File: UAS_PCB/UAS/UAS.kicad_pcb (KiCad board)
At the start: 2 copper layers, 50.8 x 47.6 mm, 17 parts, among them J1 SM02B-PASS-TBT, J2 SM02B-PASS-TBT, J3 SM02B-PASS-TBT, J4 SM02B-PASS-TBT, U1 JST-7-Pin, U10 UAS-rescue_7.5V-2.4A-Converte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, U11 JST-3-Pin, U12 Signal-Pad, U13 Signal-Pad, U2 5A-5V-Converter, U3 500mA-5V-Converter, U4 12V-StepUp-Converter, U5 TB6612FNG-Dual-Motor-Driver, U6 16_Pad_2x8_Set-UAS-cache, U7 UAS-rescue_JST-4-Pin-UAS-cache, U8 JST-7-Pin, U9 JST-3-Pin

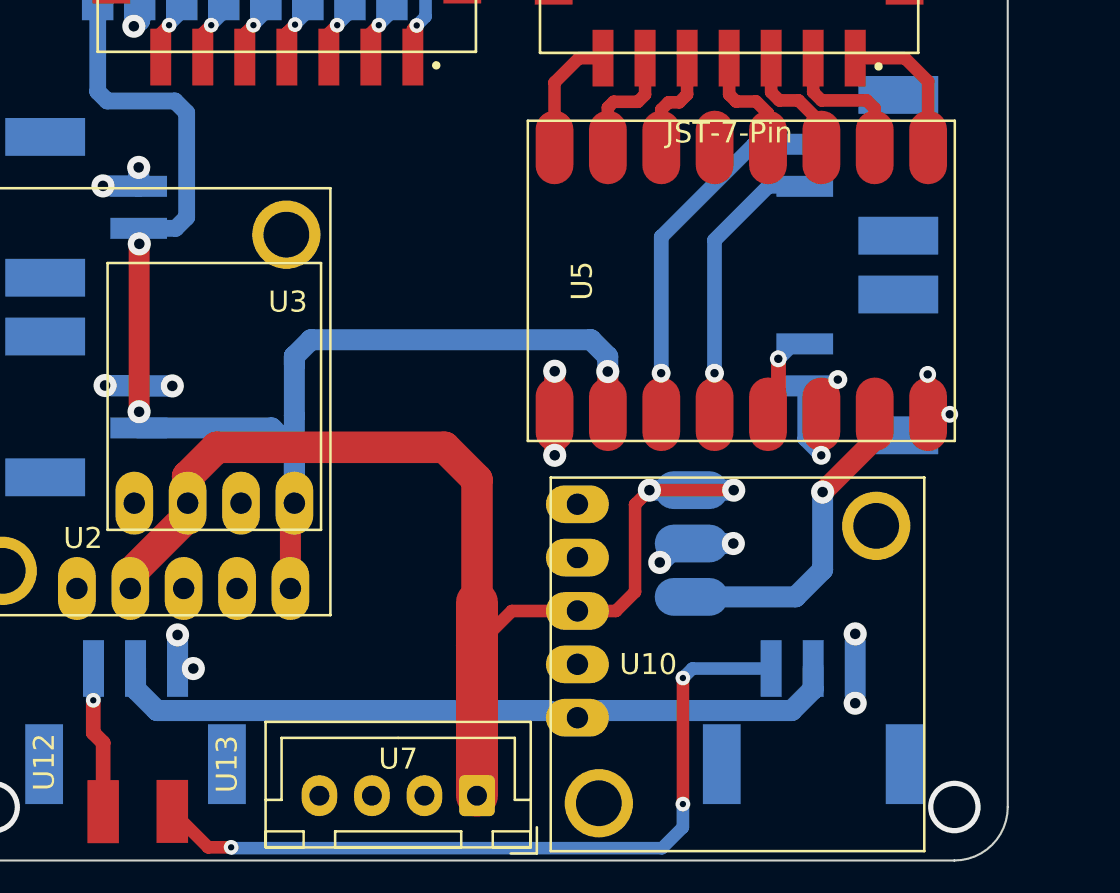
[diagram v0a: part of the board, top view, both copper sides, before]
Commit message: final version with kyles passthrough pads and graphics
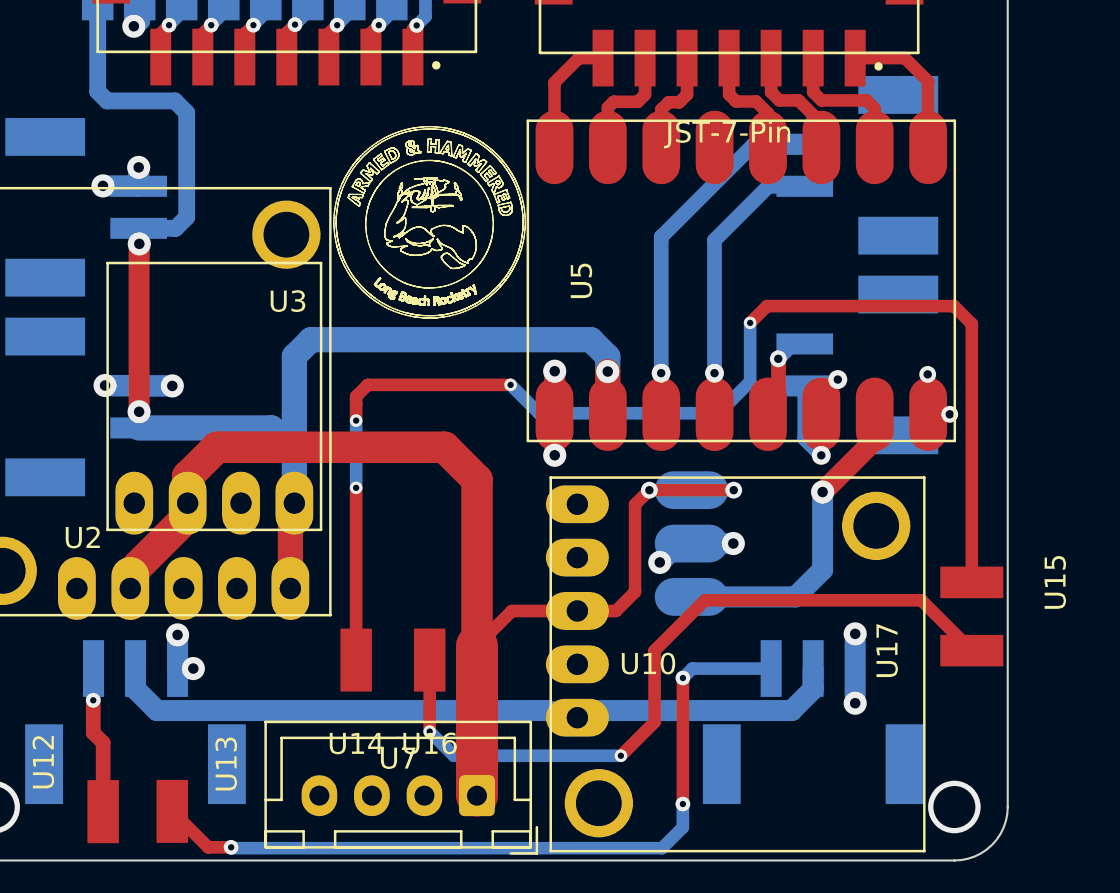
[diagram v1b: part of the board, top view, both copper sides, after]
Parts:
- added U14: UAS-rescue_Signal-Pad-UAS-cache, UAS:Individual_Solder_Pad, F.Cu at (137.2, 111.5)
- added U15: UAS-rescue_Signal-Pad-UAS-cache, UAS:Individual_Solder_Pad, F.Cu at (166.6, 107.8)
- added U16: UAS-rescue_Signal-Pad-UAS-cache, UAS:Individual_Solder_Pad, F.Cu at (140.8, 111.5)
- added U17: UAS-rescue_Signal-Pad-UAS-cache, UAS:Individual_Solder_Pad, F.Cu at (166.6, 111.1)
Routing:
- net Net-(U14-Pad1): track 0.00 -> 59.0 mm, vias 0 -> 4
- net Net-(U16-Pad1): track 0.00 -> 35.7 mm, vias 0 -> 2
